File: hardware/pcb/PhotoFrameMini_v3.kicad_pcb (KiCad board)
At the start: 2 copper layers, 42.3 x 40 mm, 31 parts, among them Q1 SI1308EDL-VB, SW1 SW_MEC_5E, U1 XIAO-nRF52840-DIP, U2 TI TPS61097A-33DBVR

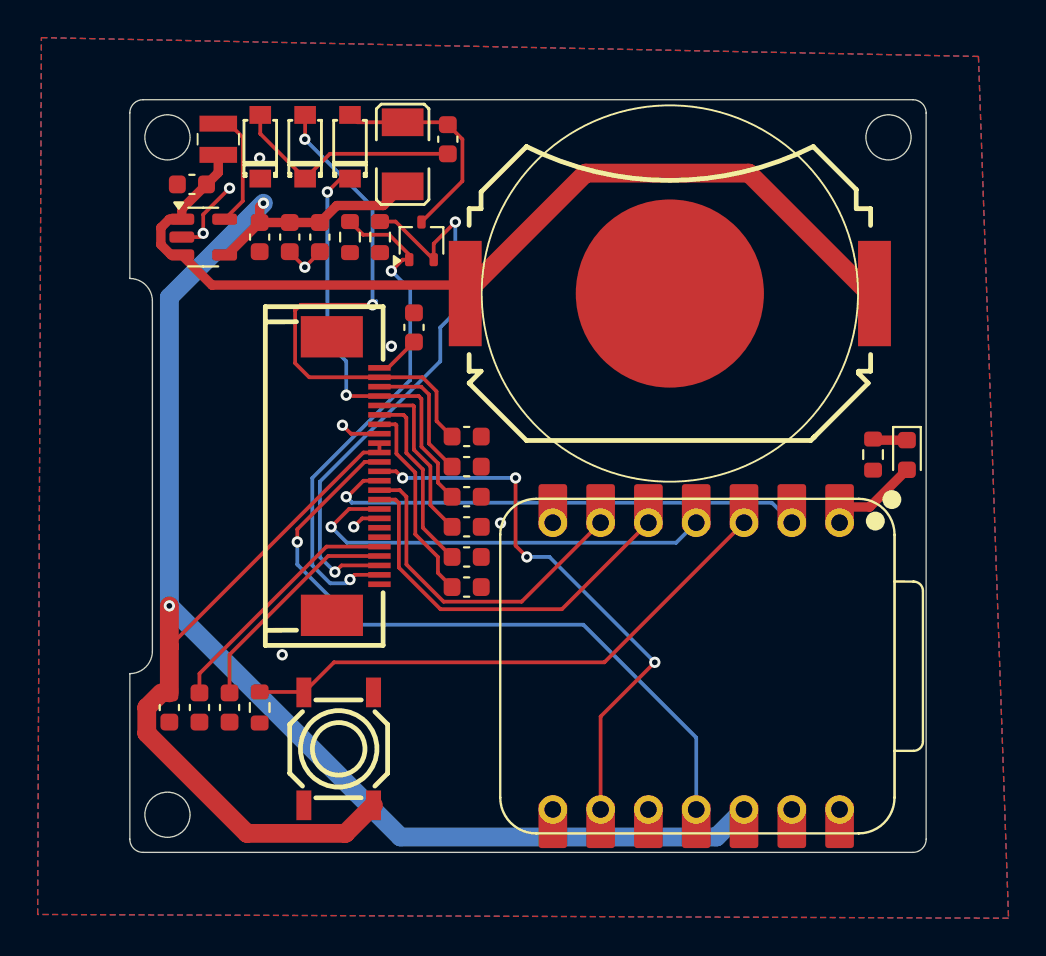
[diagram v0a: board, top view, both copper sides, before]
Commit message: update
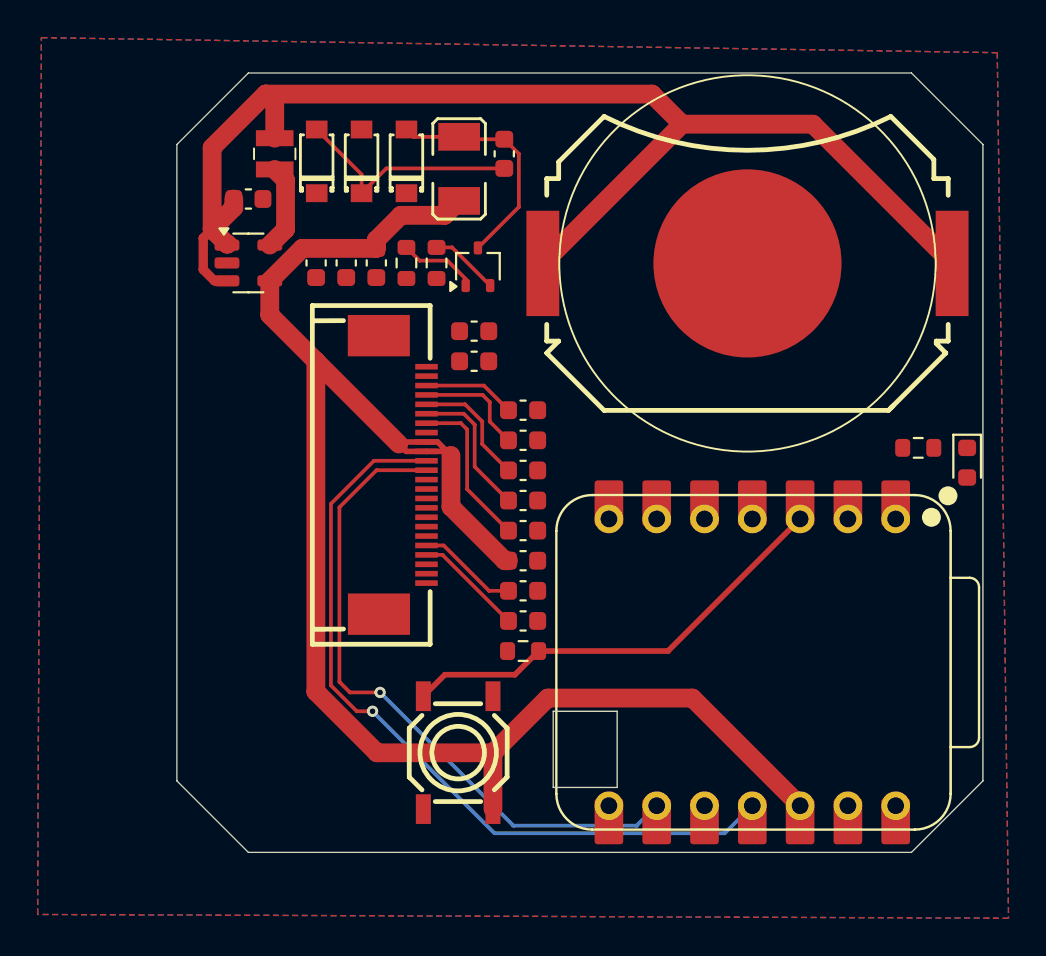
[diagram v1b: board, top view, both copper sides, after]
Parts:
- moved C6 20.4 mm to (118.4, 122.0), turned to 180 degrees
- moved C5 18.3 mm to (118.4, 123.6), turned to 180 degrees
- moved C4 16.3 mm to (118.4, 125.2), turned to 180 degrees
- moved R4 14.3 mm to (118.4, 126.8), turned to 0 degrees
- moved SW1 6.35 mm to (115.0, 132.2)
- moved BT1 4.42 mm to (130.3, 106.2)
- moved C10 4.24 mm to (118.4, 115.6)
- moved C11 4.24 mm to (118.4, 114.0)
- moved C7 4.24 mm to (118.4, 120.4)
- moved C8 4.24 mm to (118.4, 118.8)
- moved C9 4.24 mm to (118.4, 117.2)
- moved C12 4.02 mm to (115.8, 111.4)
- moved C15 3.30 mm to (107.4, 106.2)
- moved C2 3.30 mm to (110.6, 106.2)
- moved C3 3.30 mm to (109.0, 106.2)
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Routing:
- net PREVGL: track 29.8 -> 0.00 mm, vias 2 -> 0
- net RESE: track 30.6 -> 3.69 mm, vias 2 -> 0
- net CS: track 26.4 -> 0.00 mm, vias 1 -> 0
- net GDR: track 27.8 -> 4.19 mm, vias 2 -> 0
- net BUSY: track 23.1 -> 0.00 mm, vias 1 -> 0
- net 3.3V: track 110.1 -> 88.4 mm, vias 2 -> 0
- net RST: track 20.6 -> 0.00 mm
- net D/C: track 18.1 -> 0.00 mm
- net BAT: track 51.5 -> 68.7 mm
- net PREVGH: track 22.7 -> 5.96 mm, vias 2 -> 0
- net GND: track 10.2 -> 0.00 mm, vias 9 -> 0
- net Net-(C5-Pad2): track 13.4 -> 5.36 mm
- net Net-(C4-Pad2): track 12.2 -> 5.81 mm
- net Net-(SW1-K): track 29.5 -> 23.9 mm
- net SDI: track 36.5 -> 41.9 mm
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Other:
- board size 42.3 x 40 mm -> 42.8 x 41.4 mm
